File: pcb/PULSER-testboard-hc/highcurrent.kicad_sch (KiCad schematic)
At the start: 52 parts, among them Q1 N-ch, Vds>=60V, low Qgs, Q2 N-ch, Vds>=60V, low Rds, U3 LT3763

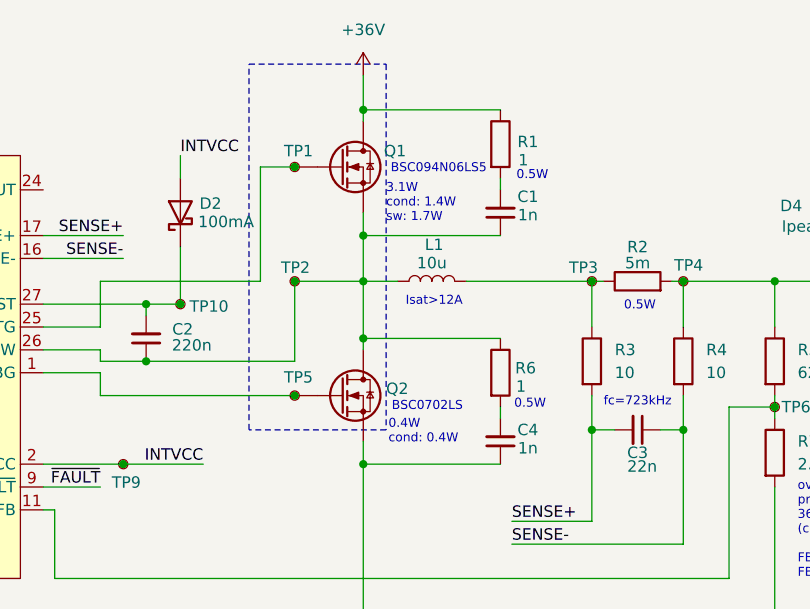
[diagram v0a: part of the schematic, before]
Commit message: HC r3 schem draft ok
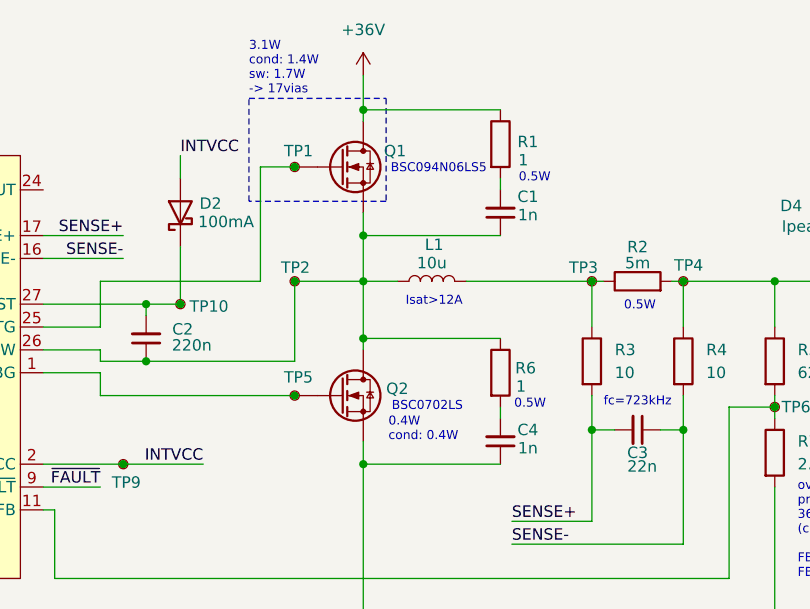
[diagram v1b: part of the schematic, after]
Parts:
- C1, C4: footprint Capacitor_SMD:C_0603_1608Metric -> Capacitor_SMD:C_0402_1005Metric; LCSC C1588 -> C1523
- C14: footprint Capacitor_SMD:C_1206_3216Metric -> Capacitor_SMD:C_0603_1608Metric; LCSC C50254 -> C23630
- C17, C18: footprint Capacitor_SMD:C_0603_1608Metric -> Capacitor_SMD:C_0402_1005Metric; LCSC C57112 -> C15195
- C2: LCSC (none) -> C21120
- C3: footprint Capacitor_SMD:C_0603_1608Metric -> Capacitor_SMD:C_0402_1005Metric; LCSC C21122 -> C1532
- C6: footprint Capacitor_SMD:C_0603_1608Metric -> Capacitor_SMD:C_0402_1005Metric; LCSC C1620 -> C26412
- C7: footprint Capacitor_SMD:C_0603_1608Metric -> Capacitor_SMD:C_0402_1005Metric; LCSC C53987 -> C1538
- R10: footprint Resistor_SMD:R_0603_1608Metric -> Resistor_SMD:R_0402_1005Metric; LCSC C25808 -> C144802
- R13, R25: footprint Resistor_SMD:R_0603_1608Metric -> Resistor_SMD:R_0402_1005Metric; LCSC C25819 -> C25792
- R26: footprint Resistor_SMD:R_0603_1608Metric -> Resistor_SMD:R_0402_1005Metric; LCSC C23159 -> C852817; Rating 72V -> 50V
- R3, R4: footprint Resistor_SMD:R_0603_1608Metric -> Resistor_SMD:R_0402_1005Metric; LCSC C22859 -> C25077
- R5: footprint Resistor_SMD:R_0603_1608Metric -> Resistor_SMD:R_0402_1005Metric; LCSC C23221 -> C423271
- R7: footprint Resistor_SMD:R_0603_1608Metric -> Resistor_SMD:R_0402_1005Metric; LCSC C13167 -> C423290
- R8: footprint Resistor_SMD:R_0603_1608Metric -> Resistor_SMD:R_0402_1005Metric; LCSC C4216 -> C728559
- R9: footprint Resistor_SMD:R_0603_1608Metric -> Resistor_SMD:R_0402_1005Metric; LCSC C23254 -> C852929
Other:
- note added: "3.1W cond: 1.4W sw: 1.7W -> 17vias"
- note removed: "3.1W cond: 1.4W sw: 1.7W"
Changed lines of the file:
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@@
 	)
 	(rectangle
-		(start 135.89 26.67)
-		(end 151.13 67.31)
+		(start 135.89 30.48)
+		(end 151.13 41.91)
 		(stroke
 			(width 0)
@@
 	(text "0.4W\ncond: 0.4W"
 		(exclude_from_sim no)
-		(at 151.384 67.564 0)
+		(at 151.384 67.31 0)
 		(effects
 			(font
@@
 		)
 	)
-	(text "3.1W\ncond: 1.4W\nsw: 1.7W"
+	(text "3.1W\ncond: 1.4W\nsw: 1.7W\n-> 17vias"
 		(exclude_from_sim no)
-		(at 151.13 42.164 0)
+		(at 135.89 27.178 0)
 		(effects
 			(font
@@
 	(text "0.5W"
 		(exclude_from_sim no)
-		(at 165.608 39.116 0)
+		(at 165.862 39.37 0)
 		(effects
 			(font
@@
 			)
 		)
-		(property "Footprint" "Capacitor_SMD:C_0603_1608Metric"
+		(property "Footprint" "Capacitor_SMD:C_0402_1005Metric"
 			(at 81.28 121.92 0)
 			(effects
@@
 			)
 		)
-		(property "LCSC" "C53987"
+		(property "LCSC" "C1538"
 			(at 81.28 121.92 0)
 			(effects
@@
 			)
 		)
-		(property "Footprint" "Resistor_SMD:R_0603_1608Metric"
+		(property "Footprint" "Resistor_SMD:R_0402_1005Metric"
 			(at 73.66 123.698 90)
 			(effects
@@
 			)
 		)
-		(property "LCSC" "C4216"
+		(property "LCSC" "C728559"
 			(at 73.66 121.92 90)
 			(effects
@@
 			)
 		)
-		(property "Footprint" "Capacitor_SMD:C_0603_1608Metric"
+		(property "Footprint" "Capacitor_SMD:C_0402_1005Metric"
 			(at 77.47 133.35 0)
 			(effects
@@
 			)
 		)
-		(property "LCSC" "C1620"
+		(property "LCSC" "C26412"
 			(at 77.47 133.35 0)
 			(effects
@@
 			)
 		)
-		(property "Footprint" "Capacitor_SMD:C_0603_1608Metric"
+		(property "Footprint" "Capacitor_SMD:C_0402_1005Metric"
 			(at 195.58 149.86 0)
 			(effects
@@
 			)
 		)
-		(property "LCSC" "C57112"
+		(property "LCSC" "C15195"
 			(at 195.58 149.86 0)
 			(effects
@@
 			)
 		)
-		(property "Footprint" "Resistor_SMD:R_0603_1608Metric"
+		(property "Footprint" "Resistor_SMD:R_0402_1005Metric"
 			(at 192.532 59.69 90)
 			(effects
@@
 			)
 		)
-		(property "LCSC" "C23221"
+		(property "LCSC" "C423271"
 			(at 194.31 59.69 0)
 			(effects
@@
 			)
 		)
-		(property "Footprint" "Resistor_SMD:R_0603_1608Metric"
+		(property "Footprint" "Resistor_SMD:R_0402_1005Metric"
 			(at 172.212 59.69 90)
 			(effects
@@
 			)
 		)
-		(property "LCSC" "C22859"
+		(property "LCSC" "C25077"
 			(at 173.99 59.69 0)
 			(effects
@@
 			)
 		)
-		(property "Footprint" "Capacitor_SMD:C_0603_1608Metric"
+		(property "Footprint" "Capacitor_SMD:C_0402_1005Metric"
 			(at 187.96 149.86 0)
 			(effects
@@
 			)
 		)
-		(property "LCSC" "C57112"
+		(property "LCSC" "C15195"
 			(at 187.96 149.86 0)
 			(effects
@@
 			)
 		)
-		(property "LCSC" ""
+		(property "LCSC" "C21120"
 			(at 124.46 57.15 0)
 			(effects
@@
 			)
 		)
-		(property "Footprint" "Capacitor_SMD:C_1206_3216Metric"
+		(property "Footprint" "Capacitor_SMD:C_0603_1608Metric"
 			(at 130.81 137.16 0)
 			(effects
@@
 			)
 		)
-		(property "LCSC" "C50254"
+		(property "LCSC" "C23630"
 			(at 130.81 137.16 0)
 			(effects
@@
 			)
 		)
-		(property "Footprint" "Resistor_SMD:R_0603_1608Metric"
+		(property "Footprint" "Resistor_SMD:R_0402_1005Metric"
 			(at 77.47 152.908 90)
 			(effects
@@
 			)
 		)
-		(property "LCSC" "C25808"
+		(property "LCSC" "C144802"
 			(at 77.47 151.13 90)
 			(effects
@@
 			)
 		)
-		(property "Footprint" "Capacitor_SMD:C_0603_1608Metric"
+		(property "Footprint" "Capacitor_SMD:C_0402_1005Metric"
 			(at 163.83 68.58 0)
 			(effects
@@
 			)
 		)
-		(property "LCSC" "C1588"
+		(property "LCSC" "C1523"
 			(at 163.83 68.58 0)
 			(effects
@@
 			)
 		)
-		(property "Footprint" "Resistor_SMD:R_0603_1608Metric"
+		(property "Footprint" "Resistor_SMD:R_0402_1005Metric"
 			(at 182.372 59.69 90)
 			(effects
@@
 			)
 		)
-		(property "LCSC" "C22859"
+		(property "LCSC" "C25077"
 			(at 184.15 59.69 0)
 			(effects
@@
 			)
 		)
-		(property "Footprint" "Capacitor_SMD:C_0603_1608Metric"
+		(property "Footprint" "Capacitor_SMD:C_0402_1005Metric"
 			(at 163.83 43.18 0)
 			(effects
@@
 			)
 		)
-		(property "LCSC" "C1588"
+		(property "LCSC" "C1523"
 			(at 163.83 43.18 0)
 			(effects
@@
 			)
 		)
-		(property "Footprint" "Resistor_SMD:R_0603_1608Metric"
+		(property "Footprint" "Resistor_SMD:R_0402_1005Metric"
 			(at 139.192 130.81 90)
 			(effects
@@
 			)
 		)
-		(property "LCSC" "C25819"
+		(property "LCSC" "C25792"
 			(at 140.97 130.81 0)
 			(effects
@@
 			)
 		)
-		(property "Footprint" "Resistor_SMD:R_0603_1608Metric"
+		(property "Footprint" "Resistor_SMD:R_0402_1005Metric"
 			(at 36.322 146.05 90)
 			(effects
@@
 			)
 		)
-		(property "LCSC" "C23159"
+		(property "LCSC" "C852817"
 			(at 38.1 146.05 0)
 			(effects
@@
 			)
 		)
-		(property "Rating" "72V"
+		(property "Rating" "50V"
 			(at 38.1 146.05 0)
 			(effects
@@
 			)
 		)
-		(property "Footprint" "Capacitor_SMD:C_0603_1608Metric"
+		(property "Footprint" "Capacitor_SMD:C_0402_1005Metric"
 			(at 179.07 67.31 0)
 			(effects
@@
 			)
 		)
-		(property "LCSC" "C21122"
+		(property "LCSC" "C1532"
 			(at 179.07 67.31 90)
 			(effects
@@
 			)
 		)
-		(property "Footprint" "Resistor_SMD:R_0603_1608Metric"
+		(property "Footprint" "Resistor_SMD:R_0402_1005Metric"
 			(at 36.322 132.08 90)
 			(effects
@@
 			)
 		)
-		(property "LCSC" "C23254"
+		(property "LCSC" "C852929"
 			(at 38.1 132.08 0)
 			(effects
@@
 			)
 		)
-		(property "Footprint" "Resistor_SMD:R_0603_1608Metric"
+		(property "Footprint" "Resistor_SMD:R_0402_1005Metric"
 			(at 116.078 135.89 90)
 			(effects
@@
 			)
 		)
-		(property "LCSC" "C25819"
+		(property "LCSC" "C25792"
 			(at 114.3 135.89 90)
 			(effects
@@
 			)
 		)
-		(property "Footprint" "Resistor_SMD:R_0603_1608Metric"
+		(property "Footprint" "Resistor_SMD:R_0402_1005Metric"
 			(at 192.532 69.85 90)
 			(effects
@@
 			)
 		)
-		(property "LCSC" "C13167"
+		(property "LCSC" "C423290"
 			(at 194.31 69.85 0)
 			(effects
